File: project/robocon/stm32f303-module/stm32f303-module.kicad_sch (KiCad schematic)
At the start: 3 parts, among them U1 STM32F303K8Tx, U2 MCP2562-E-SN, U3 NJM12888

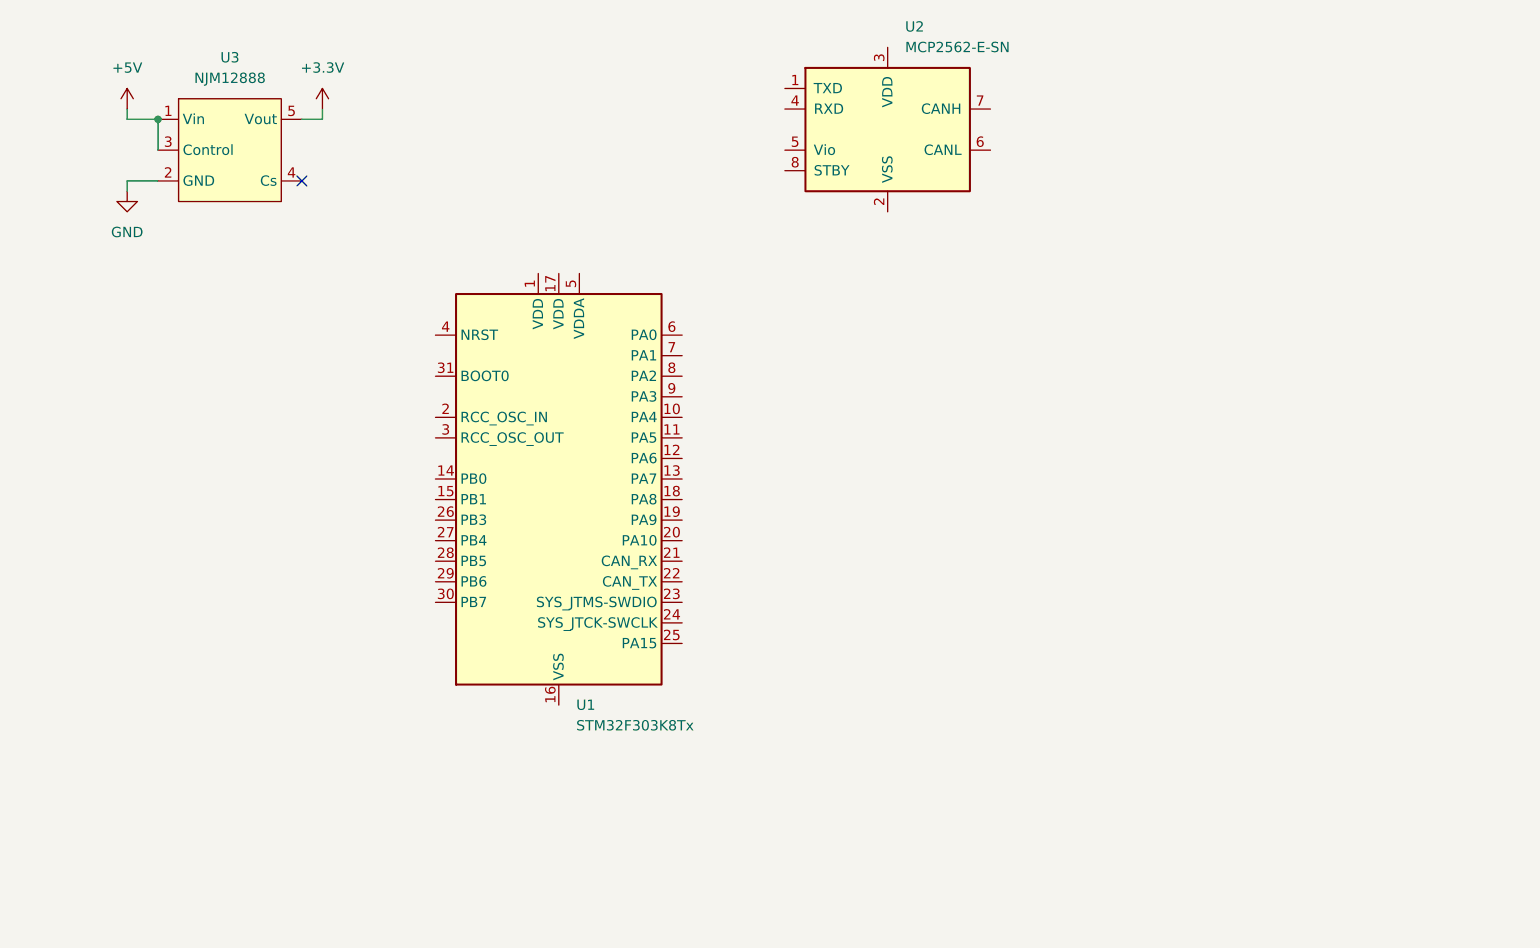
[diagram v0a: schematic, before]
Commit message: 2026/09/21/10:32
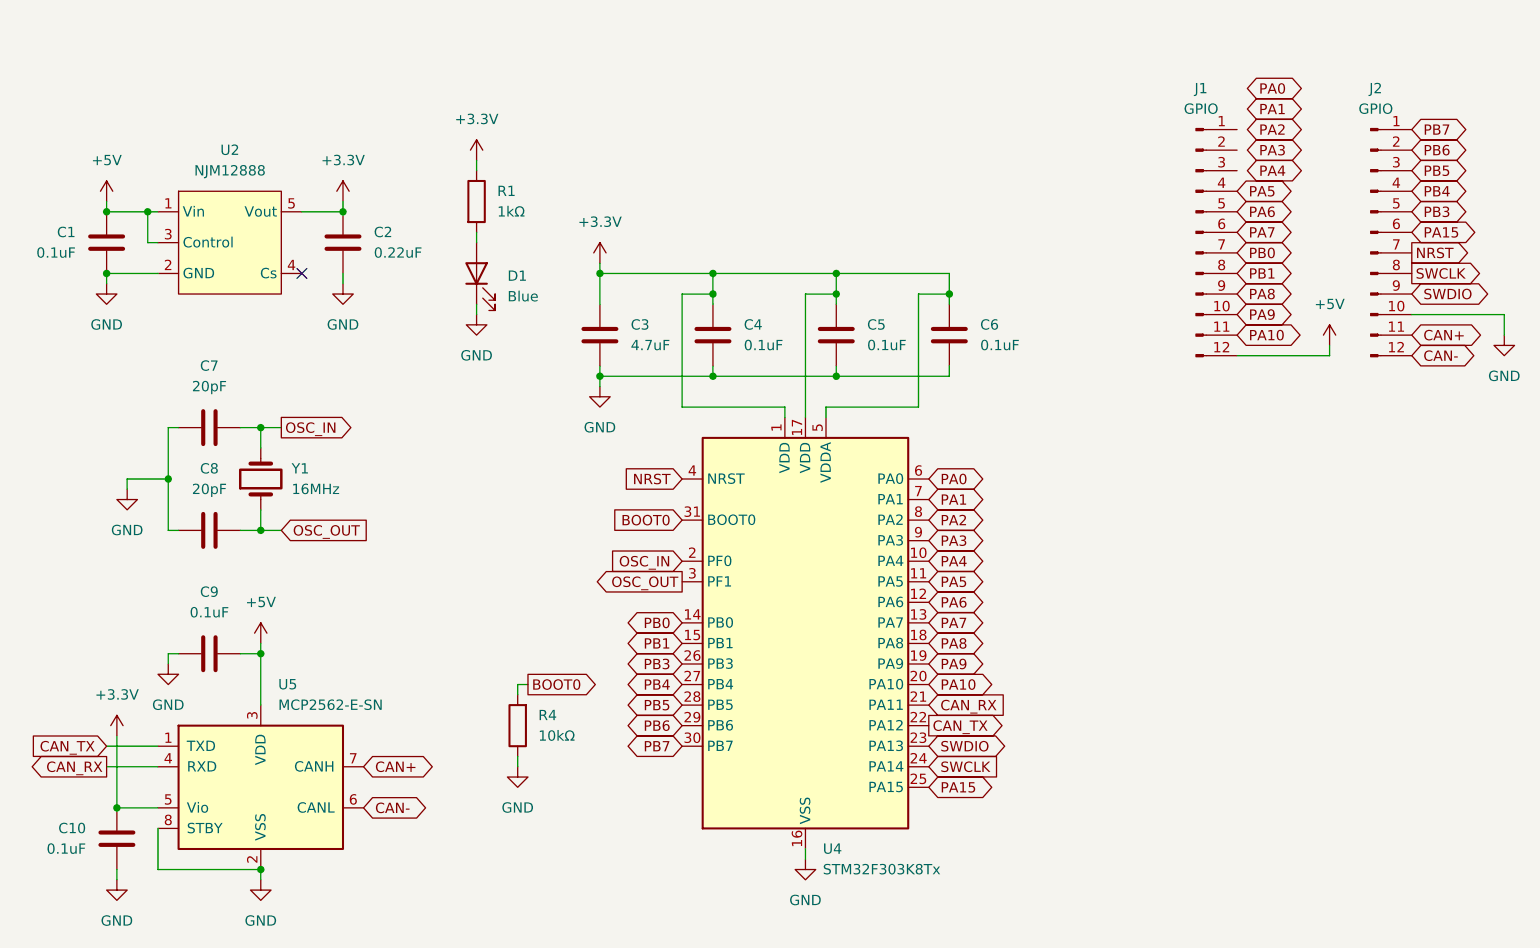
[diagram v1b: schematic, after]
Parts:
- removed U1: STM32F303K8Tx, Package_QFP:LQFP-32_7x7mm_P0.8mm, symbol MCU_ST_STM32F3:STM32F303K8Tx
- removed U2: MCP2562-E-SN, Package_SO:SOIC-8_3.9x4.9mm_P1.27mm, symbol Interface_CAN_LIN:MCP2562-E-SN
- removed U3: NJM12888, Package_TO_SOT_SMD:SOT-23-5, symbol JRC_Regulator_Linear:NJM12888F33
- added C1, C10, C4, C5, C6, C9: 0.1uF, Capacitor_SMD:C_0603_1608Metric, symbol Device:C
- added C2: 0.22uF, Capacitor_SMD:C_0603_1608Metric, symbol Device:C
- added C3: 4.7uF, Capacitor_SMD:C_0603_1608Metric, symbol Device:C
- added C7, C8: 20pF, Capacitor_SMD:C_0603_1608Metric, symbol Device:C
- added D1: Blue, LED_SMD:LED_0603_1608Metric, symbol Device:LED
- added J1, J2: GPIO, Connector_PinHeader_2.54mm:PinHeader_1x12_P2.54mm_Vertical, symbol Connector:Conn_01x12_Pin
- added R1: 1kΩ, Resistor_SMD:R_0603_1608Metric, symbol Device:R
- added R4: 10kΩ, Resistor_SMD:R_0603_1608Metric, symbol Device:R
- added U2: NJM12888, Package_TO_SOT_SMD:SOT-23-5, symbol JRC_Regulator_Linear:NJM12888F33
- added U4: STM32F303K8Tx, Package_QFP:LQFP-32_7x7mm_P0.8mm, symbol MCU_ST_STM32F3:STM32F303K8Tx
- added U5: MCP2562-E-SN, Package_SO:SOIC-8_3.9x4.9mm_P1.27mm, symbol Interface_CAN_LIN:MCP2562-E-SN
- added Y1: 16MHz, Crystal:Crystal_HC49-4H_Vertical, symbol Device:Crystal
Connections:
- net +3.3V: now also C10.1, C2.1, C3.1, C4.1, C5.1, C6.1, R1.1, U2.5 (Vout), U4.1 (VDD), U4.17 (VDD), U4.5 (VDDA), U5.5 (Vio)
- net +5V: now also C1.1, C9.2, J1.12 (Pin_12), U2.1 (Vin), U2.3 (Control), U5.3 (VDD)
- net GND: now also C1.2, C10.2, C2.2, C3.2, C4.2, C5.2, C6.2, C7.1, C8.1, C9.1, D1.1 (K), J2.10 (Pin_10), R4.1, U2.2 (GND), U4.16 (VSS), U4.32 (VSS), U5.2 (VSS), U5.8 (STBY)
- new net: D1.2 (A), R1.2
- new net BOOT0: R4.2, U4.31 (BOOT0)
- new net CAN+: J2.11 (Pin_11), U5.7 (CANH)
- new net CAN-: J2.12 (Pin_12), U5.6 (CANL)
- new net CAN_RX: U4.21 (PA11), U5.4 (RXD)
- new net CAN_TX: U4.22 (PA12), U5.1 (TXD)
- new net NRST: J2.7 (Pin_7), U4.4 (NRST)
- new net OSC_IN: C7.2, U4.2 (PF0), Y1.2
- new net OSC_OUT: C8.2, U4.3 (PF1), Y1.1
- new net PA0: U4.6 (PA0)
- new net PA1: U4.7 (PA1)
- new net PA10: J1.11 (Pin_11), U4.20 (PA10)
- new net PA15: J2.6 (Pin_6), U4.25 (PA15)
- new net PA2: U4.8 (PA2)
- new net PA3: U4.9 (PA3)
- new net PA4: U4.10 (PA4)
- new net PA5: J1.4 (Pin_4), U4.11 (PA5)
- new net PA6: J1.5 (Pin_5), U4.12 (PA6)
- new net PA7: J1.6 (Pin_6), U4.13 (PA7)
- new net PA8: J1.9 (Pin_9), U4.18 (PA8)
- new net PA9: J1.10 (Pin_10), U4.19 (PA9)
- new net PB0: J1.7 (Pin_7), U4.14 (PB0)
- new net PB1: J1.8 (Pin_8), U4.15 (PB1)
- new net PB3: J2.5 (Pin_5), U4.26 (PB3)
- new net PB4: J2.4 (Pin_4), U4.27 (PB4)
- new net PB5: J2.3 (Pin_3), U4.28 (PB5)
- new net PB6: J2.2 (Pin_2), U4.29 (PB6)
- new net PB7: J2.1 (Pin_1), U4.30 (PB7)
- new net SWCLK: J2.8 (Pin_8), U4.24 (PA14)
- new net SWDIO: J2.9 (Pin_9), U4.23 (PA13)
